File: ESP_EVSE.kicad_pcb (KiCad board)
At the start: 2 copper layers, 41.9 x 17.8 mm, 9 parts, among them J1 0V DC in 12V+, J2 PE PP, J3 UI button, J6 Conn_02x04_Odd_Even, U1 OKI-78SR-3.3_1.5-W36-C, U2 TC4427xOA

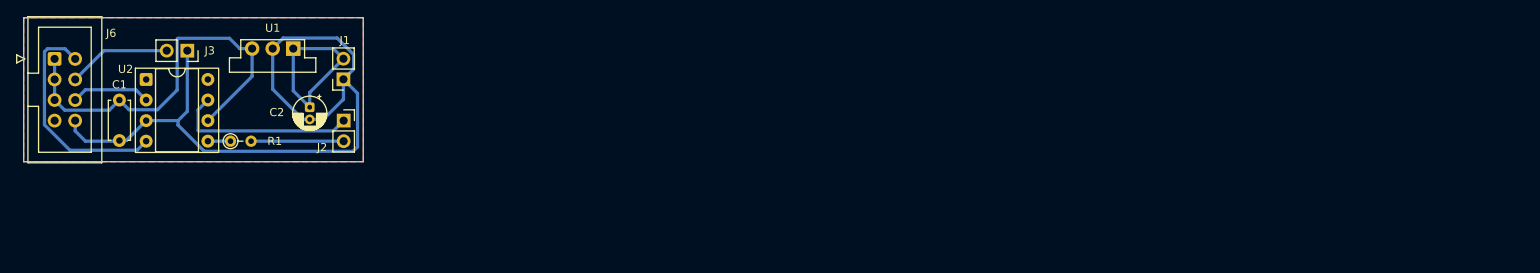
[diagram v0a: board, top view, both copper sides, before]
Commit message: Add files via upload
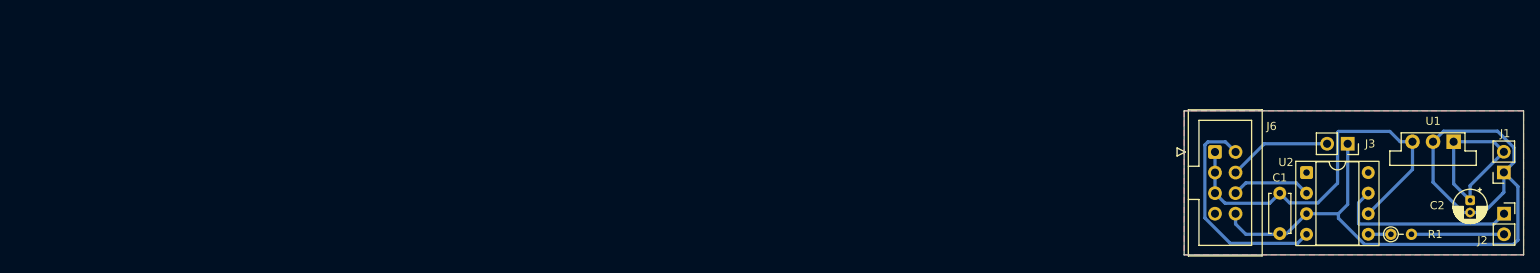
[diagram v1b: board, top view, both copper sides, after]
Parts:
- moved C2 143.7 mm to (238.3, 144.5)
- moved J2 143.7 mm to (242.4, 146.1)
- moved J3 143.7 mm to (223.1, 137.5)
- moved R1 143.7 mm to (228.5, 148.7)
- moved C1 143.7 mm to (214.8, 143.6)
- moved J1 143.7 mm to (242.4, 141.0)
- moved J6 143.7 mm to (206.8, 138.5)
- moved U1 143.7 mm to (236.2, 137.2)
- moved U2 143.7 mm to (218.1, 141.0)
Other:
- board text added: "Although the 3D models show the regulator & resistor vertical, they should be laid flat to fit under the ESP module."
